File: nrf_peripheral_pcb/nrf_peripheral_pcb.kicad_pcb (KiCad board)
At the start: 2 copper layers, 47 x 39.3 mm, 23 parts, among them U1 nRF52810-QCxx, U2 LIS2HH12, X1 32MHz

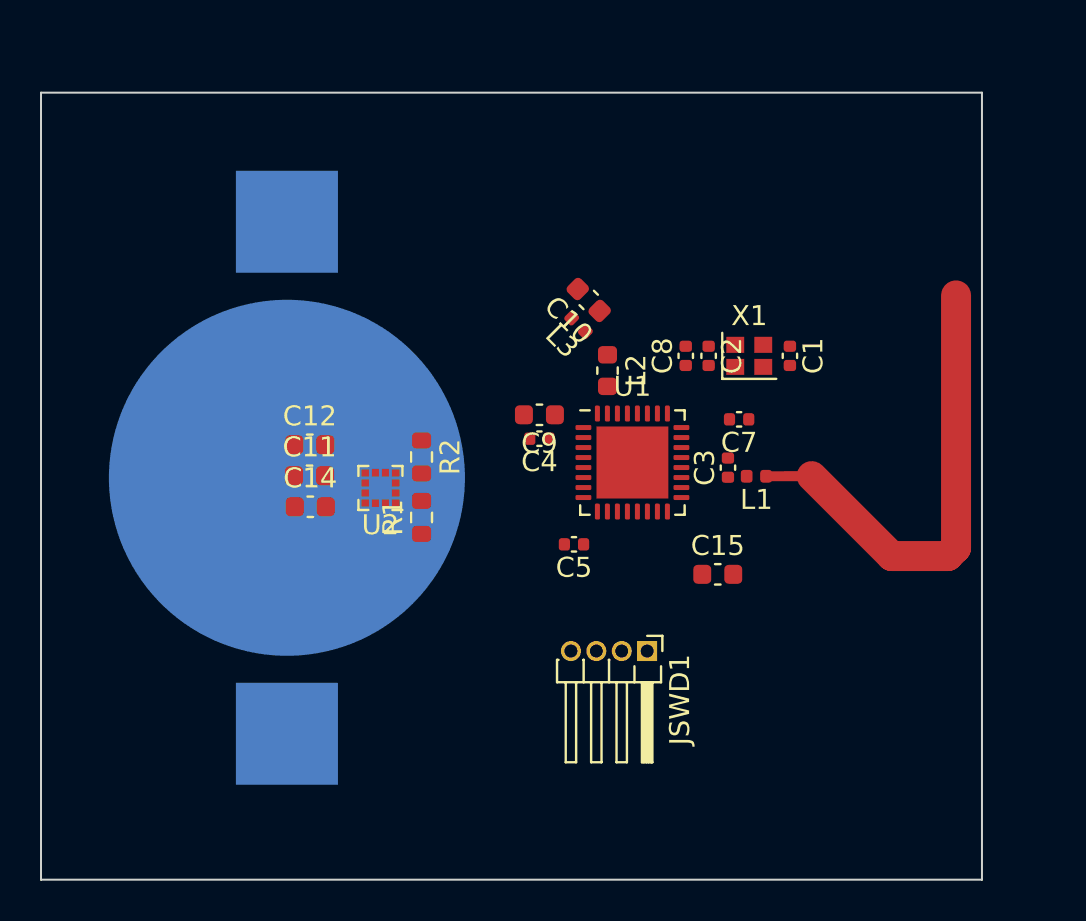
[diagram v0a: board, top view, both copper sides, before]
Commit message: pcb changes
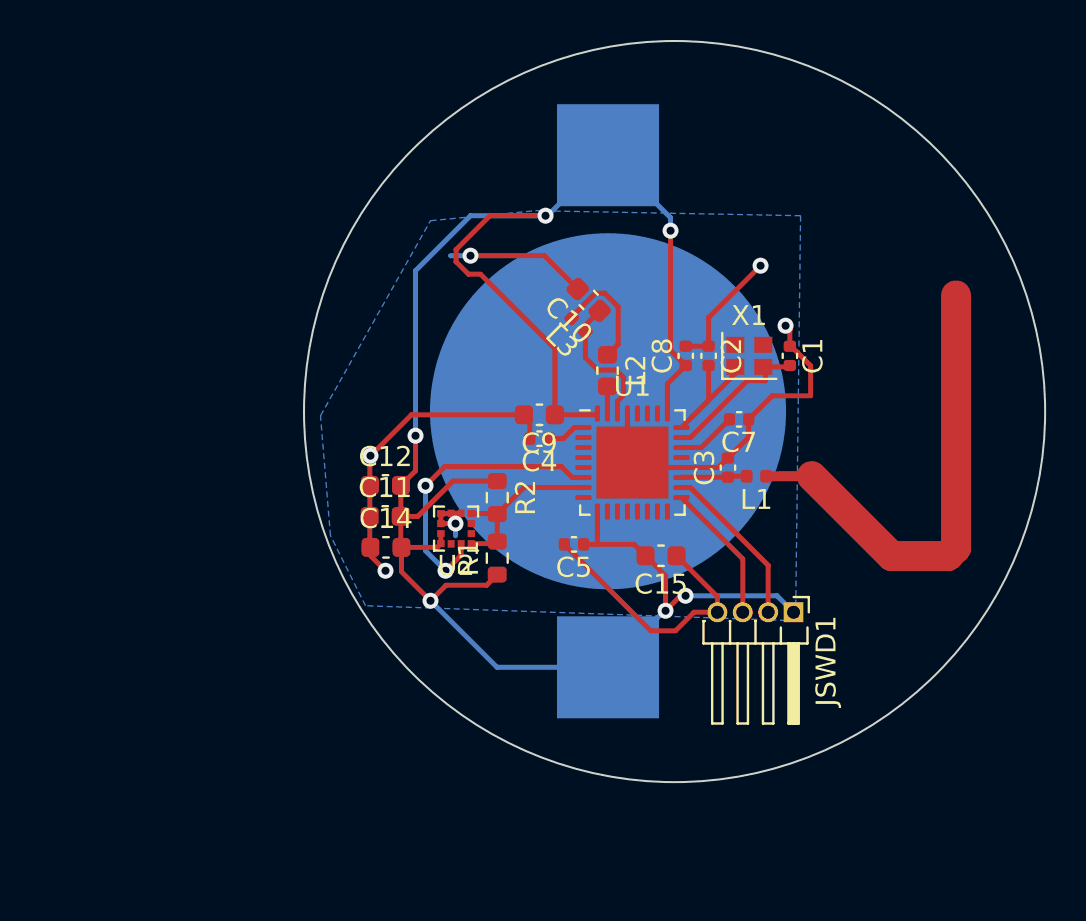
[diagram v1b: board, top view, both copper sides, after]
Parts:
- moved BT1 16.4 mm to (134.9, 104.8), turned to 90 degrees
- moved JSWD1 7.57 mm to (144.2, 114.8)
- moved R1 4.30 mm to (129.3, 112.1)
- moved R2 4.30 mm to (129.3, 109.1)
- moved C11 4.30 mm to (123.7, 110.0)
- moved C12 4.30 mm to (123.7, 108.5)
- moved C14 4.30 mm to (123.8, 111.6)
- moved U2 4.30 mm to (127.3, 110.6)
- moved C15 2.98 mm to (137.5, 112.0), turned to 180 degrees
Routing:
- net VDD_nRF: track 0.00 -> 104.6 mm, vias 0 -> 6
- net GND: track 0.00 -> 62.8 mm, vias 0 -> 6
- net IMU_INT: track 0.00 -> 14.8 mm, vias 0 -> 2
- net SDA: track 0.00 -> 8.87 mm
- net Net-(JSWD1-Pad2): track 0.00 -> 8.29 mm
- net Net-(X1-Pad2): track 0.00 -> 7.49 mm
- net Net-(X1-Pad1): track 0.00 -> 7.08 mm
- net Net-(JSWD1-Pad3): track 0.00 -> 7.00 mm
- net Net-(L3-Pad1): track 0.00 -> 6.88 mm
- net Net-(L3-Pad2): track 0.00 -> 5.77 mm
- net Net-(L1-Pad2): track 0.00 -> 3.29 mm
- net Net-(C7-Pad2): track 0.00 -> 2.99 mm
- net Net-(C4-Pad1): track 0.00 -> 1.95 mm
- net Net-(L2-Pad2): track 0.00 -> 1.36 mm
- added copper zone on B.Cu, net GND
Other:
- board size 47 x 39.3 mm -> 37.1 x 37.1 mm
